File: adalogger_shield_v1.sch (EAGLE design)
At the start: 5 parts

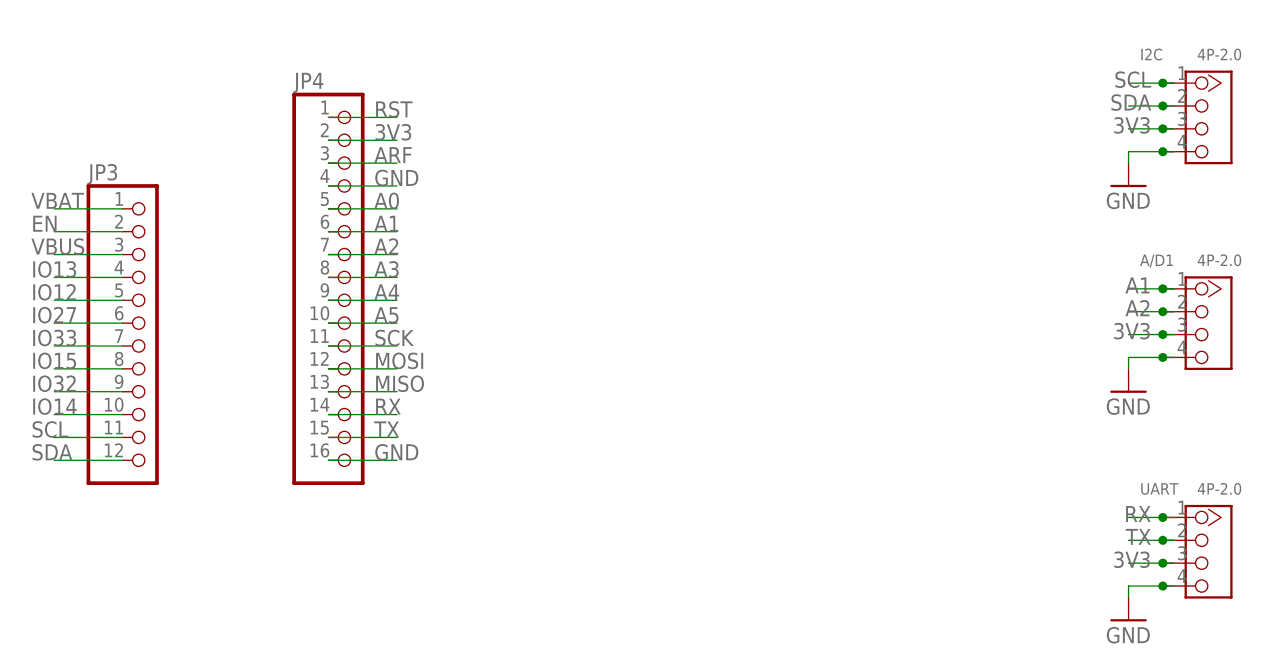
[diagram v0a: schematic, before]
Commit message: dimensions ok
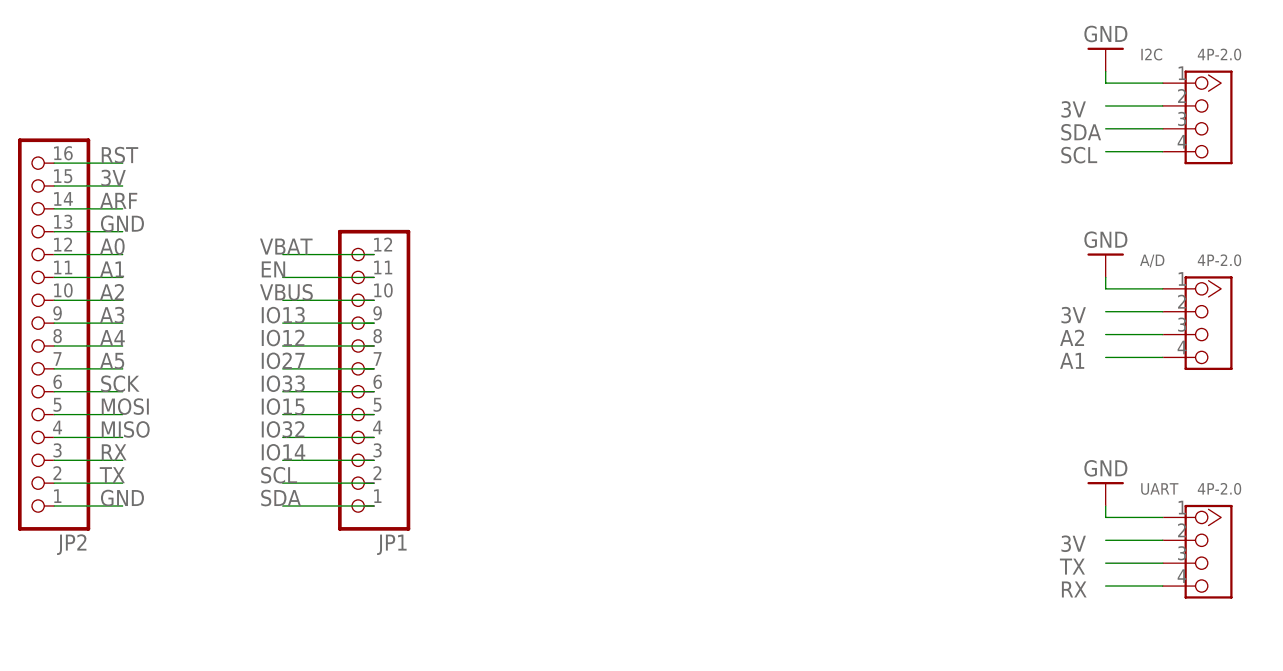
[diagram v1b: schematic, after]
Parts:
- removed JP3: (no value), pinhead:PINHD-1X12
- removed JP4: (no value), pinhead:PINHD-1X16
- added JP1: (no value), microbuilder:HEADER-1X12
- added JP2: (no value), microbuilder:HEADER-1X16ROUND
- renumbered A/D1 to A/D
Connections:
- removed net 3V3: A/D.3, I2C.3, JP4.2, UART.3
- new net 3V: A/D.2, I2C.2, JP2.15, UART.2
- net A0: now also JP2.12; no longer JP4.5
- net A1: now also A/D.4, JP2.11; no longer A/D.1, JP4.6
- net A2: now also A/D.3, JP2.10; no longer A/D.2, JP4.7
- net A3: now also JP2.9; no longer JP4.8
- net A4: now also JP2.8; no longer JP4.9
- net A5: now also JP2.7; no longer JP4.10
- net ARF: now also JP2.14; no longer JP4.3
- net EN: now also JP1.11; no longer JP3.2
- net GND: now also A/D.1, I2C.1, JP2.1, JP2.13, UART.1; no longer A/D.4, I2C.4, JP4.16, JP4.4, UART.4
- net IO12: now also JP1.8; no longer JP3.5
- net IO13: now also JP1.9; no longer JP3.4
- net IO14: now also JP1.3; no longer JP3.10
- net IO15: now also JP1.5; no longer JP3.8
- net IO27: now also JP1.7; no longer JP3.6
- net IO32: now also JP1.4; no longer JP3.9
- net IO33: now also JP1.6; no longer JP3.7
- net MISO: now also JP2.4; no longer JP4.13
- net MOSI: now also JP2.5; no longer JP4.12
- net RST: now also JP2.16; no longer JP4.1
- net RX: now also JP2.3, UART.4; no longer JP4.14, UART.1
- net SCK: now also JP2.6; no longer JP4.11
- net SCL: now also I2C.4, JP1.2; no longer I2C.1, JP3.11
- net SDA: now also I2C.3, JP1.1; no longer I2C.2, JP3.12
- net TX: now also JP2.2, UART.3; no longer JP4.15, UART.2
- net VBAT: now also JP1.12; no longer JP3.1
- net VBUS: now also JP1.10; no longer JP3.3
